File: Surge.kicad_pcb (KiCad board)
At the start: 2 copper layers, 14 parts, among them SW1 ResetSW_Neon

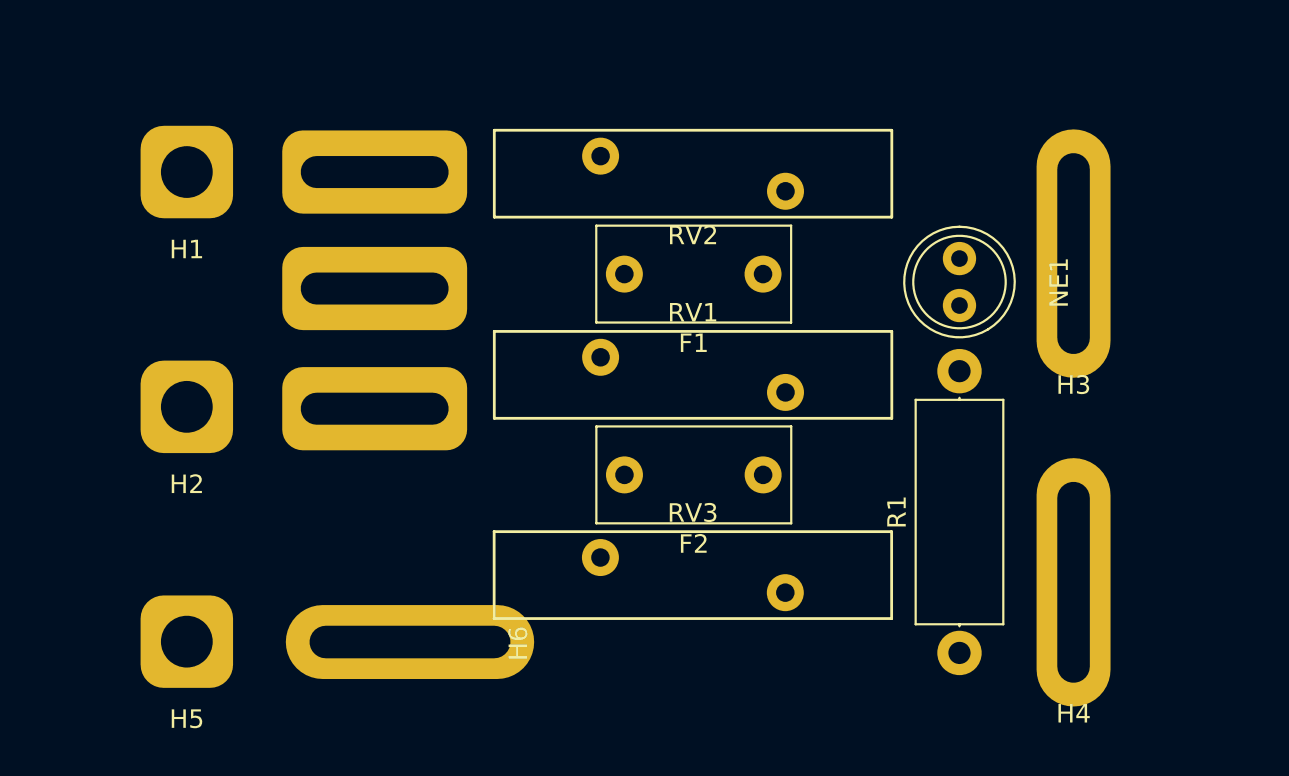
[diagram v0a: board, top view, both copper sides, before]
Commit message: Updated board layout
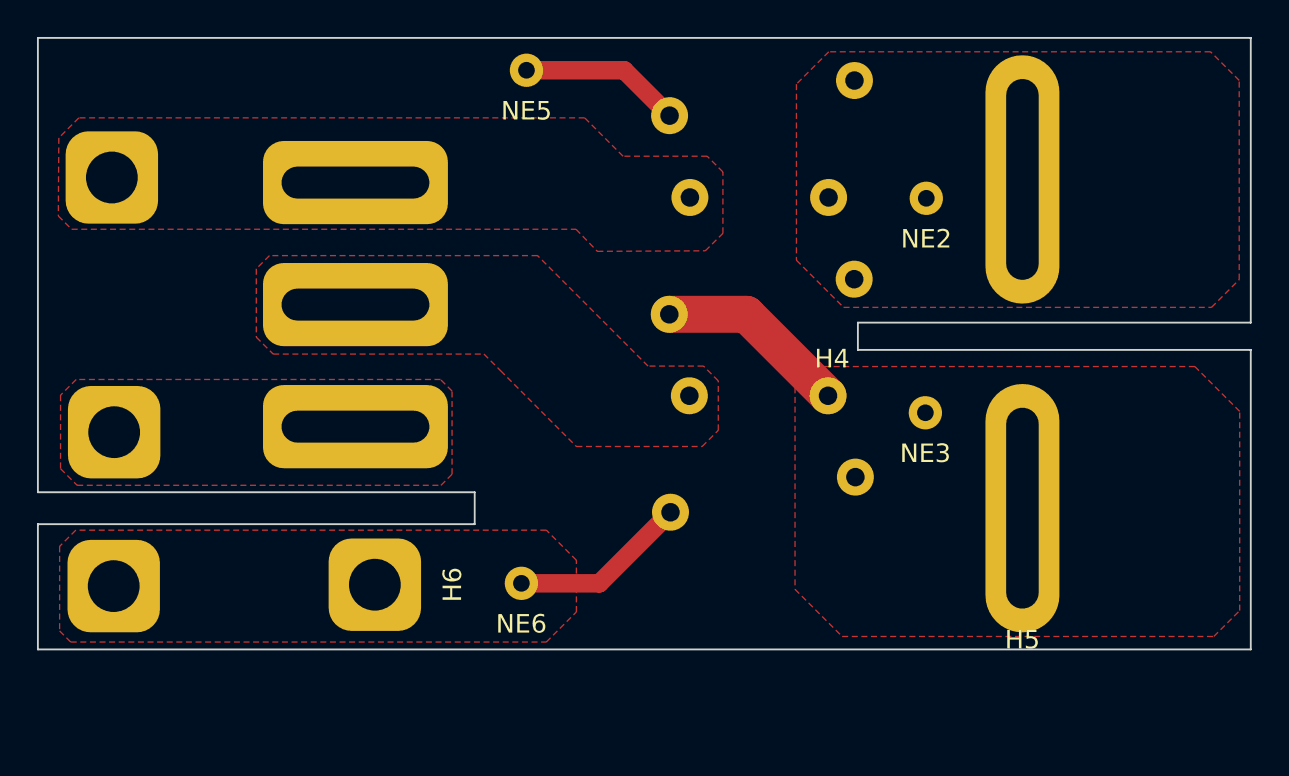
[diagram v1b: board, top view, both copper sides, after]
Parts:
- removed NE1: Lamp_Neon, Surge_Library:NE2
- removed R1: 200K Ω, Resistor_THT:R_Axial_DIN0414_L11.9mm_D4.5mm_P15.24mm_Horizontal
- added NE2: NE_N, Surge_Library:NEmount, F.Cu at (83.2, 47.3)
- added NE3: NE_L, Surge_Library:NEmount, F.Cu at (83.1, 58.9)
- added NE5: E_MOV, Surge_Library:NEmount, F.Cu at (61.5, 40.4)
- added NE6: E_E, Surge_Library:NEmount, F.Cu at (61.3, 68.1)
- F1, F2, RV3: moved to B.Cu
- H1: value L_in -> N_in
- H2: value N_in -> L_in
- H4: renamed from H3; value L_out -> N_out
- H5: renamed from H4; value N_out -> L_out
- H6: footprint Surge_Library:L_Hole -> Surge_Library:I_Hole
- RV1: renamed from RV2; moved to B.Cu
- RV2: renamed from RV1; moved to B.Cu
- moved SW1 10.2 mm to (52.3, 50.4)
- moved RV2 7.57 mm to (69.3, 50.9), turned to 0 degrees
- moved RV3 7.31 mm to (79.3, 59.7)
- moved H6 5.73 mm to (58.0, 65.5)
- moved F2 5.54 mm to (77.9, 55.3)
- moved F1 5.45 mm to (77.9, 44.6)
- moved H3 4.97 mm to (39.2, 70.3)
- moved H4 4.87 mm to (88.4, 51.2)
- moved H5 4.87 mm to (88.4, 69.0)
- moved RV1 4.33 mm to (69.3, 40.1)
- moved H2 4.16 mm to (39.2, 62.0)
- moved H1 4.07 mm to (39.1, 48.2)
- renumbered H5 to H3
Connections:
- RV1 pad 1: Earth -> Net-(NE5-Pad1)
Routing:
- net Net-(F2-Pad1): track 0.00 -> 10.4 mm
- net Earth: track 0.00 -> 9.66 mm
- net Net-(NE5-Pad1): track 0.00 -> 8.76 mm
- net Net-(SW1A-B): track 4.09 -> 0.00 mm
- added copper zone on F.Cu, net Earth
- added copper zone on F.Cu, net Net-(F1-Pad1)
- added copper zone on F.Cu, net Net-(F2-Pad1)
- added copper zone on F.Cu, net Net-(SW1A-A)
- added copper zone on F.Cu, net Net-(SW1A-B)
- added copper zone on F.Cu, net Net-(SW1A-C)
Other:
- board outline added: 65.6 x 33.1 mm
- board text added: "L Out"
- board text added: "N Out"

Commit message: Updated board layout
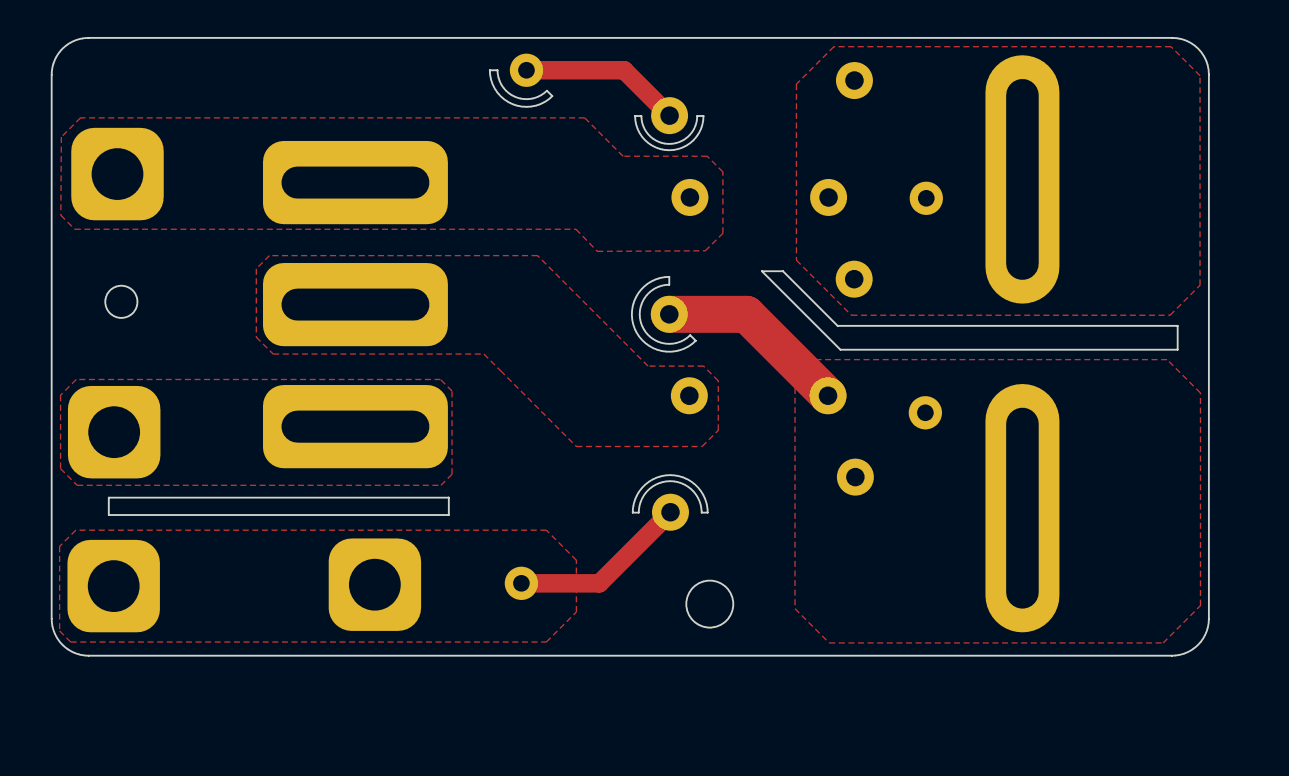
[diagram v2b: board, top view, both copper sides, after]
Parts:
- moved H1 0.36 mm to (39.4, 48.0)
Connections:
- RV1 pad 1: Net-(NE5-Pad1) -> Net-(F1-Pad1)
- RV1 pad 2: Net-(F1-Pad1) -> Net-(NE5-Pad1)
- RV2 pad 1: Net-(F2-Pad1) -> Net-(F1-Pad1)
- RV2 pad 2: Net-(F1-Pad1) -> Net-(F2-Pad1)
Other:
- board size 65.6 x 33.1 mm -> 62.6 x 33.4 mm
- board text added: "E"
- board text added: "E_Out"
- board text added: "E_Pass1"
- board text added: "E_Pass2"
- board text added: "Fuse_L"
- board text added: "Fuse_N"
- board text added: "L"
- board text added: "M2"
- board text added: "MOV1"
- board text added: "MOV2"
- board text added: "MOV3"
- board text added: "N"
- board text added: "NE1"
- board text added: "NE2"
- board text added: "SPST_Neon SW"
- board text added: "github.com/RandomDelta6 Surge 1U HC SRG04012024 Rev.001"
